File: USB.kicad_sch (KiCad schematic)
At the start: 13 parts, among them J6 USB_B_Micro, U1 FT230XS-R

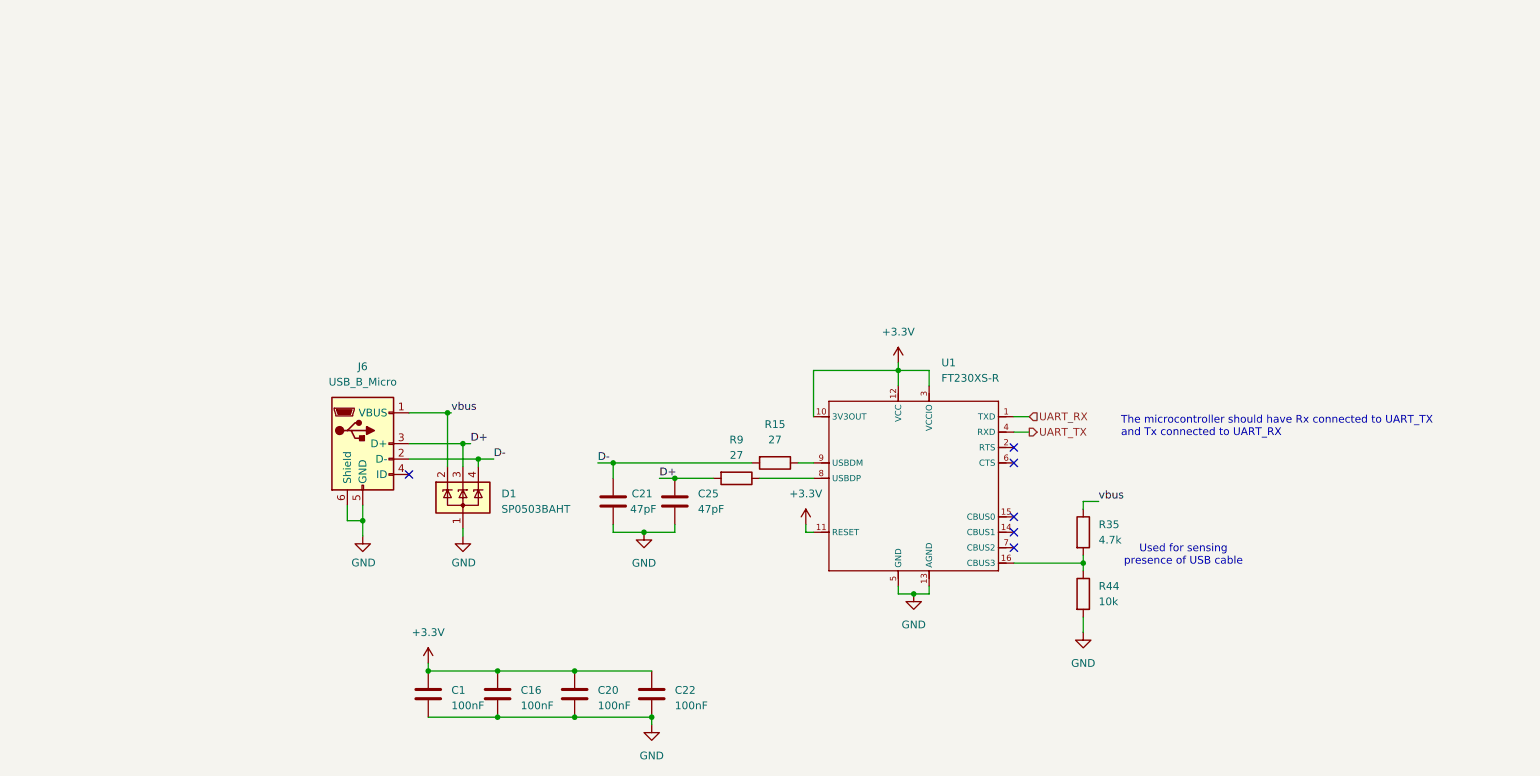
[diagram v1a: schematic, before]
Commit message: hi again lakshay
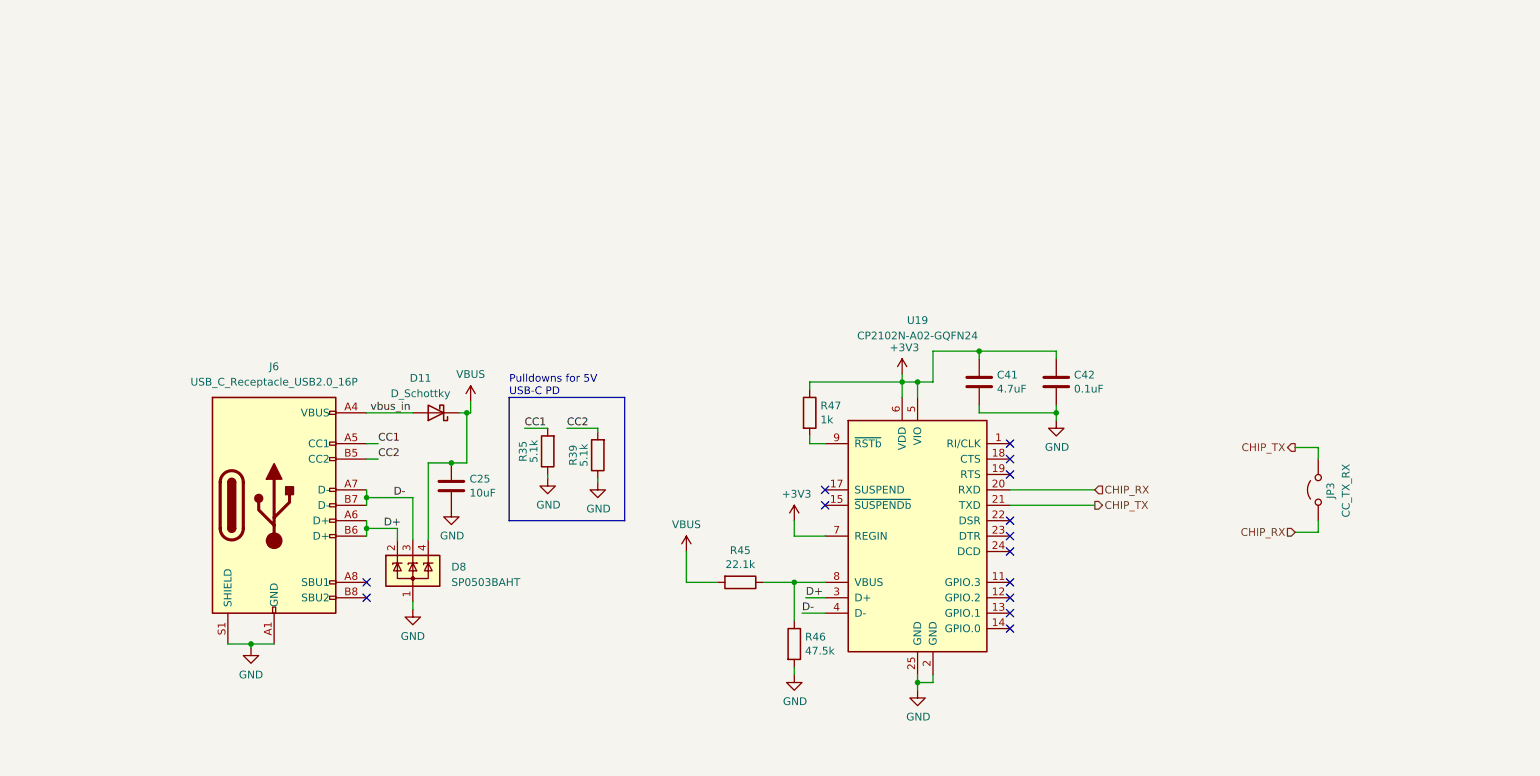
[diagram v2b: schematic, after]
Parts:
- removed C1, C16, C20, C22: 100nF, Capacitor_SMD:C_0805_2012Metric, symbol Device:C
- removed C21: 47pF, Capacitor_SMD:C_0805_2012Metric, symbol Device:C
- removed D1: SP0503BAHT, Package_TO_SOT_SMD:SOT-143, symbol utsvt-chips:SP0503BAHT-Power_Protection
- removed J6: USB_B_Micro, Connector_USB:USB_Micro-B_Molex-105017-0001, symbol Connector:USB_B_Micro
- removed R15, R9: 27, Resistor_SMD:R_0805_2012Metric, symbol Device:R
- removed R44: 10k, Resistor_SMD:R_0805_2012Metric, symbol Device:R
- removed U1: FT230XS-R, Package_SO:SSOP-16_3.9x4.9mm_P0.635mm, symbol utsvt-chips:FT230XS-R
- added C41: 4.7uF, Capacitor_SMD:C_0805_2012Metric, symbol Device:C
- added C42: 0.1uF, Capacitor_SMD:C_0805_2012Metric, symbol Device:C
- added D11: D_Schottky, Diode_SMD:D_SOD-323_HandSoldering, symbol Device:D_Schottky
- added D8: SP0503BAHT, Package_TO_SOT_SMD:SOT-143, symbol utsvt-chips:SP0503BAHT-Power_Protection
- added J6: USB_C_Receptacle_USB2.0_16P, Connector_USB:USB_C_Receptacle_GCT_USB4105-xx-A_16P_TopMnt_Horizontal, symbol Connector:USB_C_Receptacle_USB2.0_16P
- added JP3: CC_TX_RX, Connector_PinHeader_2.54mm:PinHeader_1x02_P2.54mm_Vertical, symbol Jumper:Jumper_2_Open
- added R39: 5.1k, Resistor_SMD:R_0805_2012Metric, symbol Device:R
- added R45: 22.1k, Resistor_SMD:R_0805_2012Metric, symbol Device:R
- added R46: 47.5k, Resistor_SMD:R_0805_2012Metric, symbol Device:R
- added R47: 1k, Resistor_SMD:R_0805_2012Metric, symbol Device:R
- added U19: CP2102N-A02-GQFN24, Package_DFN_QFN:QFN-24-1EP_4x4mm_P0.5mm_EP2.6x2.6mm, symbol Interface_USB:CP2102N-A01-GQFN24
- C25: value 47pF -> 10uF; Mouser Part Number (none) -> 581-22201C106KAT2A; P/N (none) -> TMK212BBJ106MGHT
- R35: value 4.7k -> 5.1k
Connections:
- net vbus is gone; now on net GND: R35.1
- net D+: now also D8.2 (K), J6.A6 (D+), J6.B6 (D+), U19.3 (D+); no longer C25.1
- net D-: now also D8.3 (K), J6.A7 (D-), J6.B7 (D-), U19.4 (D-)
- net GND: now also C41.2, C42.2, D8.1 (A), J6.A1 (GND), J6.A12 (GND), J6.B1 (GND), J6.B12 (GND), J6.S1 (SHIELD), R39.1, R46.2, U19.2 (GND), U19.25 (GND)
- net CC1: now reaches R35.2
- net CC1: now also J6.A5 (CC1)
- new net: R45.1, R46.1, U19.8 (VBUS)
- new net: R47.2, U19.9 (~{RSTb})
- new net +3V3: C41.1, C42.1, R47.1, U19.5 (VIO), U19.6 (VDD), U19.7 (REGIN)
- new net CC2: J6.B5 (CC2), R39.2
- new net CHIP_RX: JP3.1 (A), U19.20 (RXD)
- new net CHIP_TX: JP3.2 (B), U19.21 (TXD)
- new net VBUS: C25.1, D11.1 (K), D8.4 (K), R45.2
- new net vbus_in: D11.2 (A), J6.A4 (VBUS), J6.A9 (VBUS), J6.B4 (VBUS), J6.B9 (VBUS)
- no-connect marks 6 -> 14
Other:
- note added: "Pulldowns for 5V USB-C PD"
- note removed: "The microcontroller should have Rx connected to UART_TX and Tx connected to UART_RX"
- note removed: "Used for sensing presence of USB cable"

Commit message: MCU pins, PSON power distribution, KiCad-Sharepoint, and 7 seg
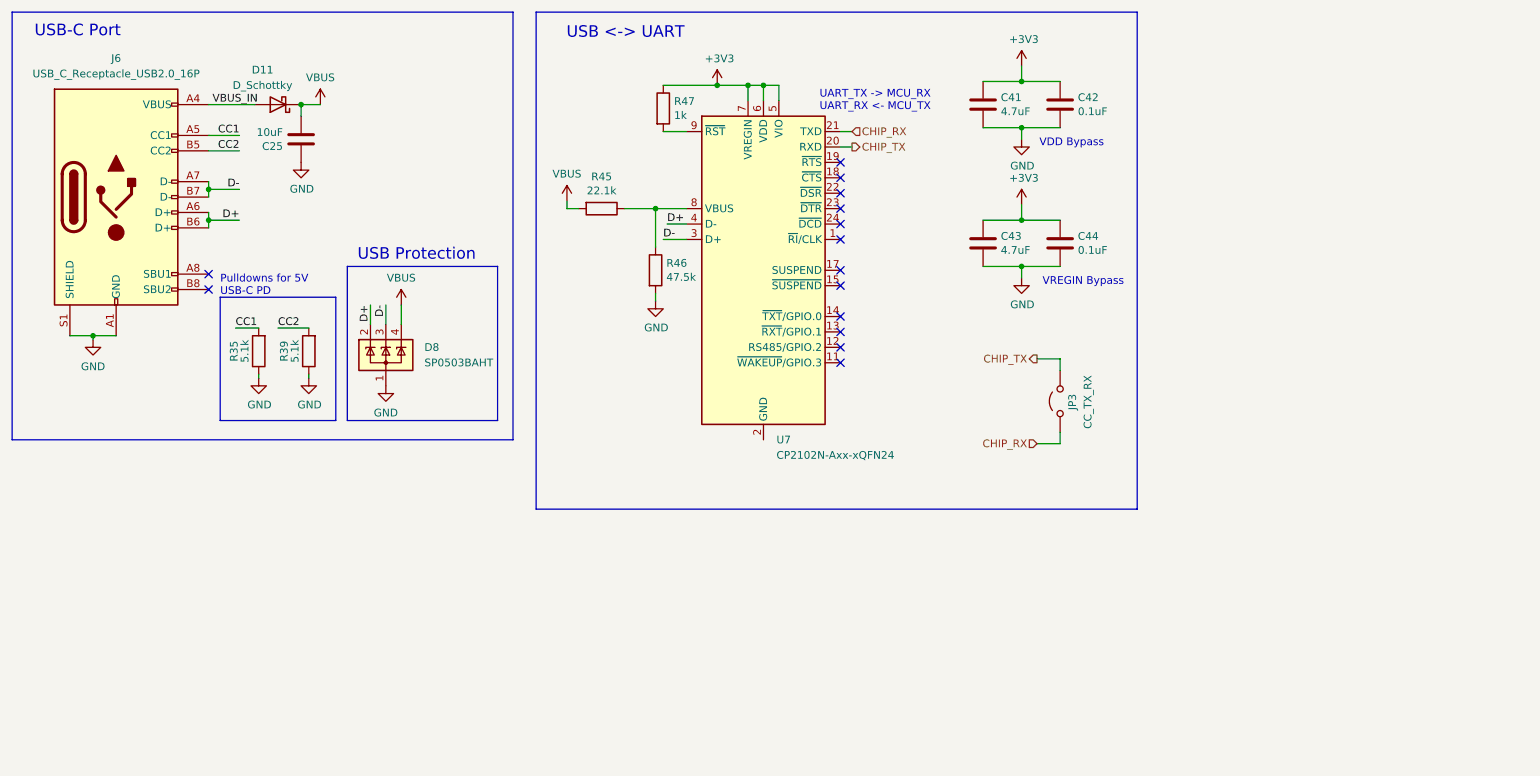
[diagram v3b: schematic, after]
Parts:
- removed U19: CP2102N-A02-GQFN24, Package_DFN_QFN:QFN-24-1EP_4x4mm_P0.5mm_EP2.6x2.6mm, symbol Interface_USB:CP2102N-A01-GQFN24
- added C43: 4.7uF, Capacitor_SMD:C_0805_2012Metric, symbol Device:C
- added C44: 0.1uF, Capacitor_SMD:C_0805_2012Metric, symbol Device:C
- added U7: CP2102N-Axx-xQFN24, UTSVT_ICs:CP2102N-A02-GQFN24, symbol UTSVT-ICs:CP2102N-Axx-xQFN24
- D8: symbol utsvt-chips:SP0503BAHT-Power_Protection -> UTSVT-ICs:SP0503BAH
- J6: footprint Connector_USB:USB_C_Receptacle_GCT_USB4105-xx-A_16P_TopMnt_Horizontal -> UTSVT_ICs:USB_C_Receptacle_GCT_USB4105-xx-A_16P_TopMnt_Horizontal; symbol Connector:USB_C_Receptacle_USB2.0_16P -> UTSVT-Connectors:USB_C_Receptacle_USB2.0_16P
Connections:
- net +3V3: now also C43.1, C44.1, U7.5 (VIO), U7.6 (VDD), U7.7 (VREGIN)
- net CHIP_RX: now also U7.21 (TXD)
- net CHIP_TX: now also U7.20 (RXD)
- net D+: now also U7.4 (D-)
- net D-: now also U7.3 (D+)
- net GND: now also C25.1, J6.S2 (Shield), J6.S3 (Shield), J6.S4 (Shield), C43.2, C44.2; no longer C25.2
- net VBUS: now also C25.2; no longer C25.1
- net at R45.1, R46.1: now also U7.8 (VBUS)
- net at R47.2: now also U7.9 (~{RST})
- net vbus_in renamed VBUS_IN
- new net: U7.2 (GND), U7.25 (GND)
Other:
- note added: "UART_TX -> MCU_RX UART_RX <- MCU_TX"
- note added: "USB <-> UART"
- note added: "USB Protection"
- note added: "USB-C Port"
- note added: "VDD Bypass"
- note added: "VREGIN Bypass"
- moved on the sheet: C25, C41, C42, D11, D8, JP3, R35, R39, R45, R46, R47
